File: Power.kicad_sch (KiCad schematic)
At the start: 30 parts, among them IC1 LM74502HDDFR, IC2 LM74502HDDFR, Q3 PSMN8R5-40MSDX, Q4 PSMN8R5-40MSDX

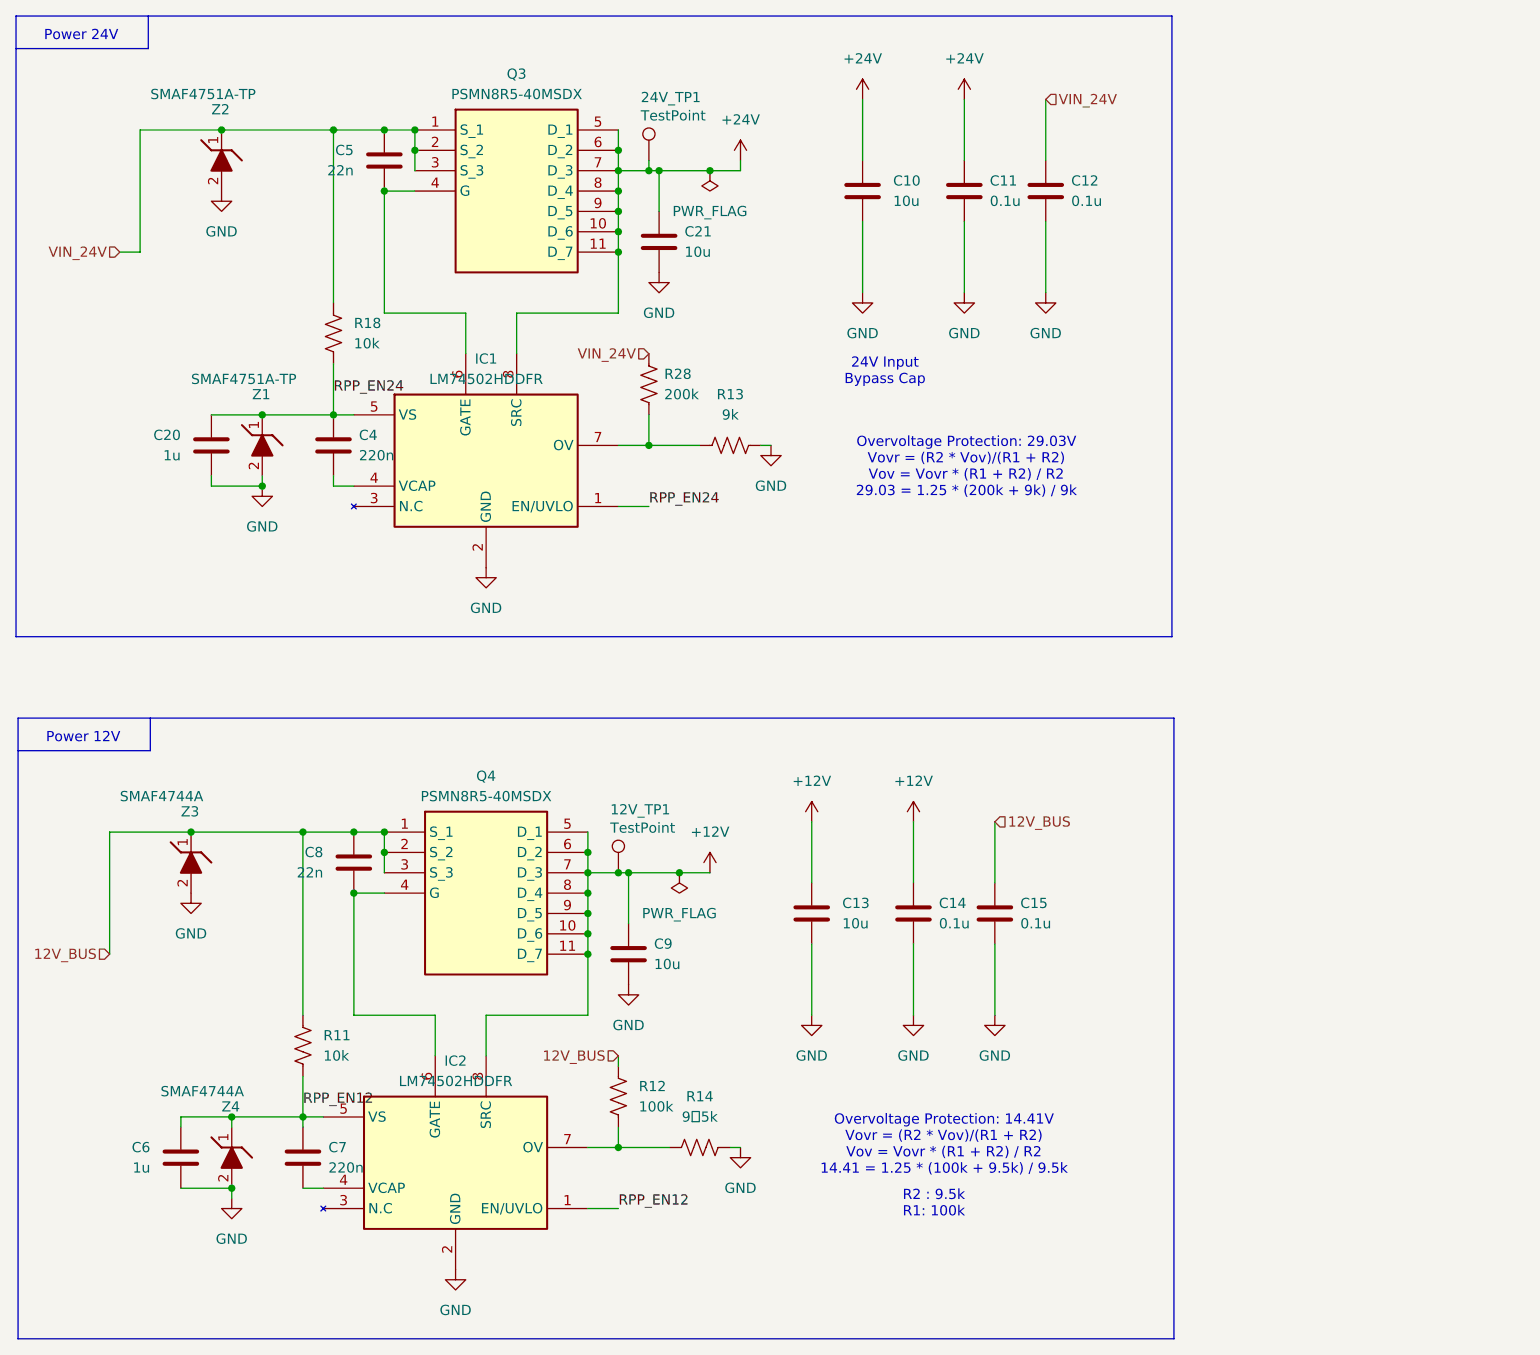
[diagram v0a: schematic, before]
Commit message: changes + ioc
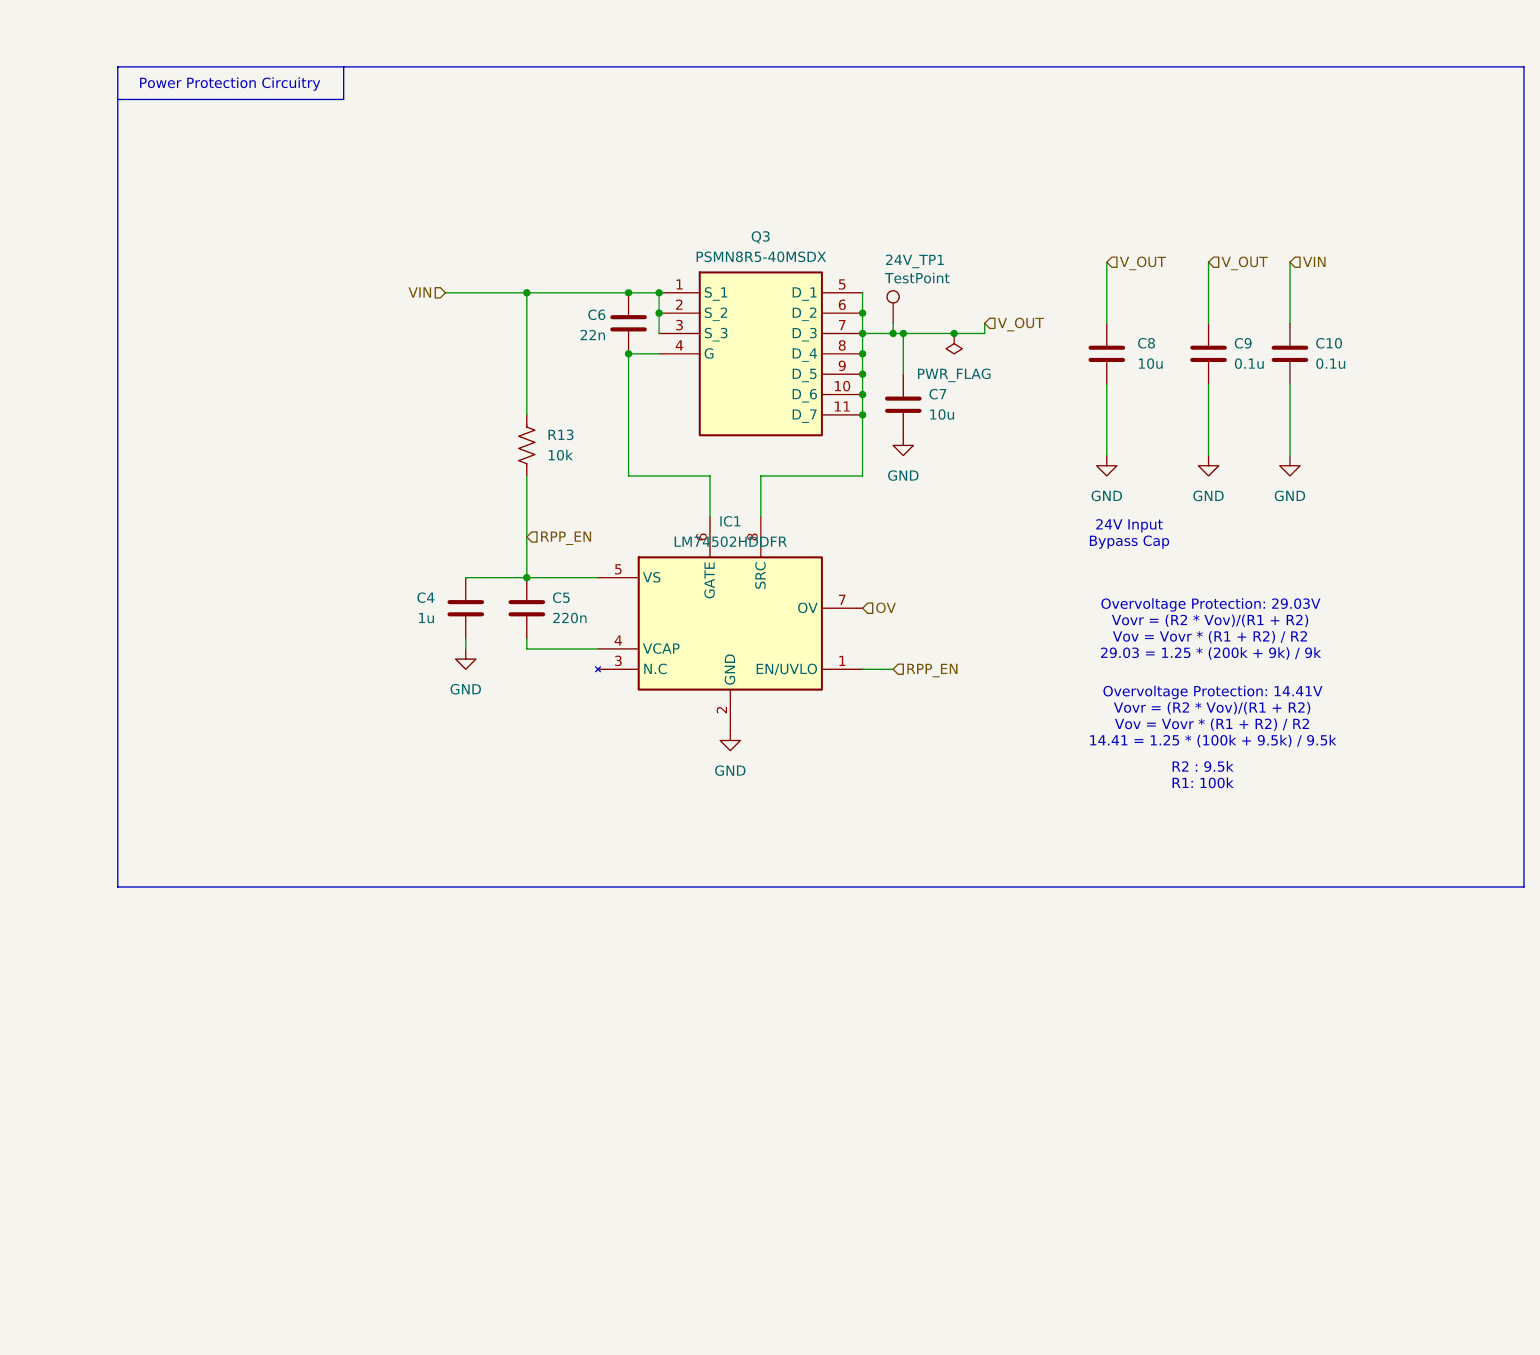
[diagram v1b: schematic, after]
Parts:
- removed 12V_TP1: TestPoint, UTSVT_Special:TestPoint_HEX_3mmID, symbol Connector:TestPoint
- removed C11, C12, C14, C15: 0.1u, Capacitor_SMD:C_0603_1608Metric, symbol Device:C
- removed C13, C21: 10u, Capacitor_SMD:C_0805_2012Metric, symbol Device:C
- removed C20: 1u, Capacitor_SMD:C_0603_1608Metric, symbol Device:C
- removed IC2: LM74502HDDFR, UTSVT_Power:SOT65P280X110-8N, symbol UTSVT_ICs:LM74502HDDFR
- removed Q4: PSMN8R5-40MSDX, UTSVT_Power:PSMN8R5-40MSDX, symbol UTSVT_Power:PSMN8R5-40MSDX
- removed R11, R18: 10k, Resistor_SMD:R_0603_1608Metric, symbol Device:R_US
- removed R12: 100k, Resistor_SMD:R_0603_1608Metric, symbol Device:R_US
- removed R14: 9。5k, Resistor_SMD:R_0603_1608Metric, symbol Device:R_US
- removed R28: 200k, Resistor_SMD:R_0603_1608Metric, symbol Device:R_US
- removed Z1, Z2: SMAF4751A-TP, UTSVT_Passives:SODFL5026X125N, symbol UTSVT_Power:SMAF4749A-TP
- removed Z3, Z4: SMAF4744A, UTSVT_Passives:SODFL5026X125N, symbol UTSVT_Power:SMAF4749A-TP
- C10, C9: value 10u -> 0.1u; footprint Capacitor_SMD:C_0805_2012Metric -> Capacitor_SMD:C_0603_1608Metric
- C4: value 220n -> 1u
- C5: value 22n -> 220n
- C6: value 1u -> 22n
- C7: value 220n -> 10u; footprint Capacitor_SMD:C_0603_1608Metric -> Capacitor_SMD:C_0805_2012Metric
- C8: value 22n -> 10u; footprint Capacitor_SMD:C_0603_1608Metric -> Capacitor_SMD:C_0805_2012Metric
- R13: value 9k -> 10k
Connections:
- net +12V is gone; now on net V_OUT: C9.1
- net 12V_BUS is gone; now on net GND: C8.2
- net GND: now also C4.1, C7.2; no longer C6.1, R13.2
- net at IC1.4 (VCAP): now also C5.2; no longer C4.2
- net at IC1.6 (GATE), Q3.4 (G): now also C6.1; no longer C5.1
- net OV: now reaches IC1.7 (OV)
- net OV: no longer R13.1
- net V_OUT: now reaches C8.1
- net V_OUT: now also 24V_TP1.1, C7.1, IC1.8 (SRC), Q3.10 (D_6), Q3.11 (D_7), Q3.5 (D_1), Q3.6 (D_2), Q3.7 (D_3), Q3.8 (D_4), Q3.9 (D_5)
- removed net +24V: 24V_TP1.1, C10.1, IC1.8 (SRC), Q3.10 (D_6), Q3.11 (D_7), Q3.5 (D_1), Q3.6 (D_2), Q3.7 (D_3), Q3.8 (D_4), Q3.9 (D_5)
- net RPP_EN12 renamed VIN
- net VIN: now also C10.1, Q3.1 (S_1), Q3.2 (S_2), Q3.3 (S_3), R13.1; no longer C7.1
- net RPP_EN24 renamed RPP_EN
- net RPP_EN: now also C4.2, C5.1, R13.2; no longer C4.1
- removed net VIN_24V: C5.2, Q3.1 (S_1), Q3.2 (S_2), Q3.3 (S_3)
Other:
- note added: "Power Protection Circuitry"
- note removed: "Power 12V"
- note removed: "Power 24V"
